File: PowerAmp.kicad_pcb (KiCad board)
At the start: 2 copper layers, 156 parts, among them IC1 NJM4580D-D, IC2 NJM4580D-D, K1 Conn_01x02_Pin, K2 Conn_01x02_Pin, K3 Conn_01x04_Pin, K4 Conn_01x03_Pin, Q1 2SA1376-K/U, Q10 2SA1145-Y, Q11 2SC2705-Y, Q12 2SC2705-Y, Q13 2SA1145-Y, Q14 2SA1145-Y, Q15 2SC2705-Y, Q16 2SC2705-Y, Q17 2SA1507-S/T, Q18 2SC3902-S/T, Q19 2SC4793, Q2 2SA1376-K/U, Q20 2SA1837, Q21 2SC5949-O, Q22 2SA2121-O, Q23 2SC5949-O, Q24 2SA2121-O, Q25 2SC4685, Q26 2SA1376-K/U, Q27 2SC3478-K/U, Q3 2SC3478-K/U, Q4 2SC3478-K/U, Q5 2SC3478-K/U, Q6 2SC3478-K/U, Q7 2SA1376-K/U, Q8 2SA1376-K/U, Q9 2SA1145-Y

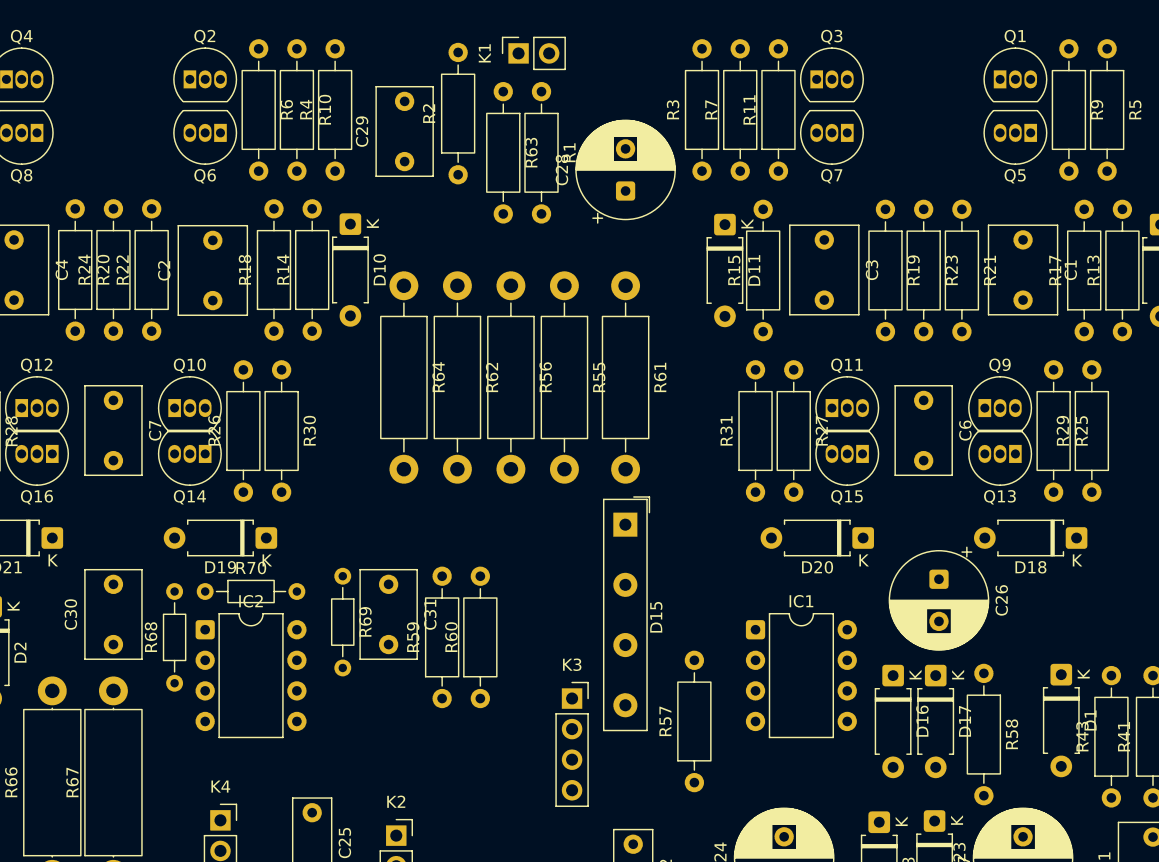
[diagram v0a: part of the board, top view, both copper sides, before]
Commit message: PCB routing
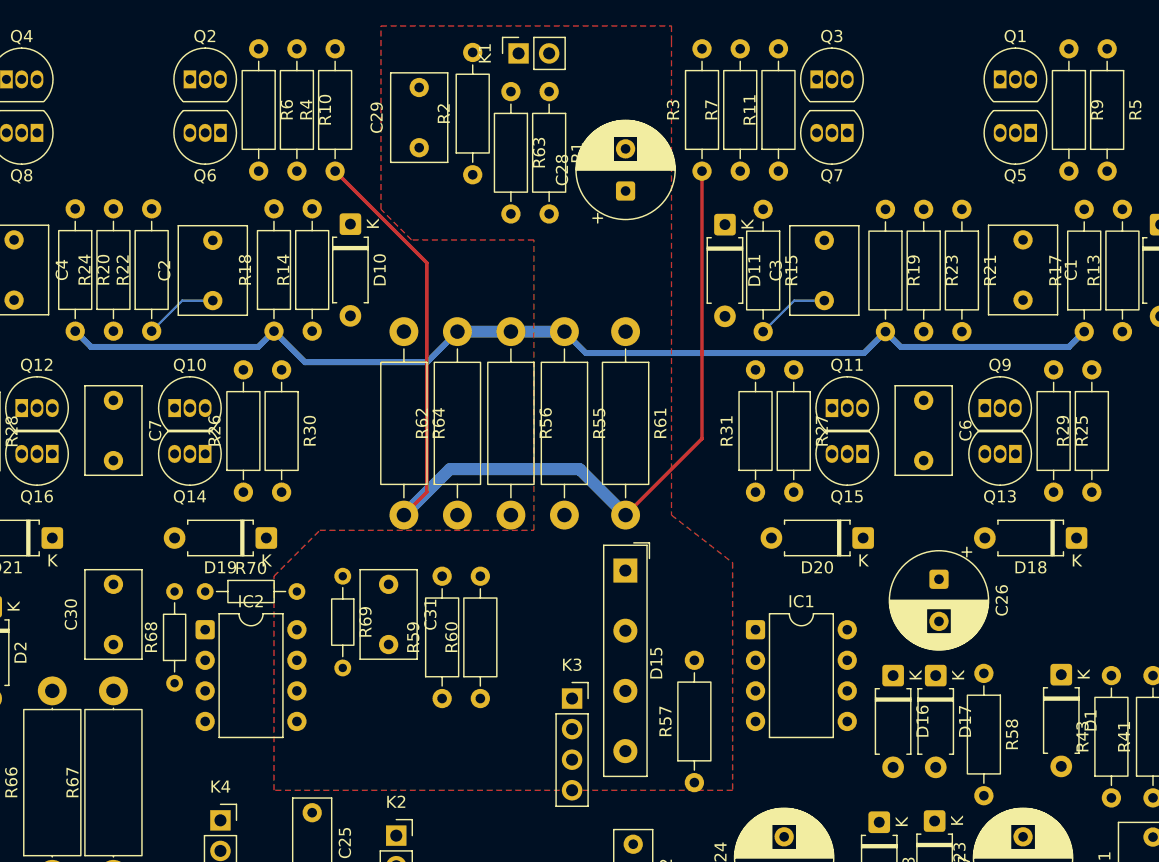
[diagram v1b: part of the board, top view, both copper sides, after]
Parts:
- moved R62 19.1 mm to (-5.08, 191.8), turned to 90 degrees
- moved R15 10.2 mm to (20.3, 166.4), turned to -90 degrees
- moved C3 5.04 mm to (25.4, 173.9), turned to 90 degrees
- moved D15 3.81 mm to (8.87, 196.4)
- moved R55 3.81 mm to (3.81, 176.5)
- moved R56 3.81 mm to (-0.64, 176.5)
- moved R61 3.81 mm to (8.89, 176.5)
- moved R64 3.81 mm to (-9.53, 176.5)
- moved C29 1.67 mm to (-8.26, 161.2)
- moved R2 1.21 mm to (-3.81, 163.5)
- moved R1 0.64 mm to (2.54, 156.6)
- moved R63 0.64 mm to (-0.64, 156.6)
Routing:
- net Net-(R17-Pad1): track 0.00 -> 89.6 mm
- net Net-(R3-Pad1): track 0.00 -> 85.3 mm
- net Net-(D20-K): track 0.00 -> 6.15 mm
- net Net-(C2-Pad1): track 0.00 -> 6.13 mm
- added copper zone on F.Cu, net GND
